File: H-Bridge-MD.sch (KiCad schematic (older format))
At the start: 70 parts, among them IC1 SI8650AB-B-IS1, IC2 AP7381-50SA-7, IC3 A3921KLPTR-T, IC4 SI8650AB-B-IS1, IC5 A3921KLPTR-T, J1 Conn_01x03, J2 Conn_01x05, J3 Bus_mechaken_PCIexpress_x16_1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, J4 Conn_01x02, J5 Conn_01x02, Q1 NVMFD5C446NT1G, Q2 NVMFD5C446NT1G, Q3 NVMFD5C446NT1G, Q4 NVMFD5C446NT1G, U1 LDL1117S33R_SOT223-4, U2 STM32F042K6Tx, U3 MCP2562-E-SN

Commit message: fix
細かな修正
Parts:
- IC2: footprint SamacSys_Parts:SOT96P240X105-3N -> SOT96P240X105-3N; symbol SamacSys_Parts:AP7381-50SA-7 -> H-Bridge-MD-rescue:AP7381-50SA-7-SamacSys_Parts
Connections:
- net MD_3V3 renamed VDD
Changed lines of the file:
@@
 Text GLabel 7600 8550 3    50   Input ~ 0
 MD_FF2_1
-Text GLabel 12750 4150 0    50   Output ~ 0
-MD_3V3
 Text Label 4800 3600 0    50   ~ 0
 CAN_TD
@@
 	0    -1   -1   0
 $EndComp
-Text GLabel 10250 3900 2    50   Input ~ 0
-MD_3V3
-Text GLabel 6050 7450 2    50   Input ~ 0
-MD_3V3
 Connection ~ 9850 10100
 Wire Wire Line
@@
 	1    0    0    -1
 $EndComp
-Text GLabel 11200 4100 3    50   Output ~ 0
-MD_3V3
 Text GLabel 11050 5100 1    50   Input ~ 0
 VREG_0
@@
 Connection ~ 11850 5000
 $Comp
-L SamacSys_Parts:AP7381-50SA-7 IC2
+L H-Bridge-MD-rescue:AP7381-50SA-7-SamacSys_Parts IC2
 U 1 1 5E271866
 P 13300 4050
 F 0 "IC2" H 13850 4315 50  0000 C CNN
 F 1 "AP7381-50SA-7" H 13850 4224 50  0000 C CNN
-F 2 "SamacSys_Parts:SOT96P240X105-3N" H 14250 4150 50  0001 L CNN
+F 2 "SOT96P240X105-3N" H 14250 4150 50  0001 L CNN
 F 3 "https://componentsearchengine.com/Datasheets/1/AP7381-50SA-7.pdf" H 14250 4050 50  0001 L CNN
 F 4 "LDO Voltage Regulators LDO CMOS LowCurr SOT23 T&R 3K" H 14250 3950 50  0001 L CNN "Description"
@@
 Wire Wire Line
 	13100 4450 14400 4450
-Wire Wire Line
-	14400 4450 14400 4050
 Connection ~ 14400 4450
+Wire Wire Line
+	14400 4050 14400 4450
+$Comp
+L power:VDD #PWR0101
+U 1 1 5E33BBA2
+P 11200 4100
+F 0 "#PWR0101" H 11200 3950 50  0001 C CNN
+F 1 "VDD" H 11217 4273 50  0000 C CNN
+F 2 "" H 11200 4100 50  0001 C CNN
+F 3 "" H 11200 4100 50  0001 C CNN
+	1    11200 4100
+	-1   0    0    1
+$EndComp
+$Comp
+L power:VDD #PWR0102
+U 1 1 5E35E290
+P 12750 4150
+F 0 "#PWR0102" H 12750 4000 50  0001 C CNN
+F 1 "VDD" H 12767 4323 50  0000 C CNN
+F 2 "" H 12750 4150 50  0001 C CNN
+F 3 "" H 12750 4150 50  0001 C CNN
+	1    12750 4150
+	0    -1   -1   0
+$EndComp
+$Comp
+L power:VDD #PWR0103
+U 1 1 5E3654B8
+P 10250 3900
+F 0 "#PWR0103" H 10250 3750 50  0001 C CNN
+F 1 "VDD" H 10267 4073 50  0000 C CNN
+F 2 "" H 10250 3900 50  0001 C CNN
+F 3 "" H 10250 3900 50  0001 C CNN
+	1    10250 3900
+	1    0    0    -1
+$EndComp
+$Comp
+L power:VDD #PWR0104
+U 1 1 5E36C54F
+P 6050 7450
+F 0 "#PWR0104" H 6050 7300 50  0001 C CNN
+F 1 "VDD" H 6067 7623 50  0000 C CNN
+F 2 "" H 6050 7450 50  0001 C CNN
+F 3 "" H 6050 7450 50  0001 C CNN
+	1    6050 7450
+	1    0    0    -1
+$EndComp
 $EndSCHEMATC

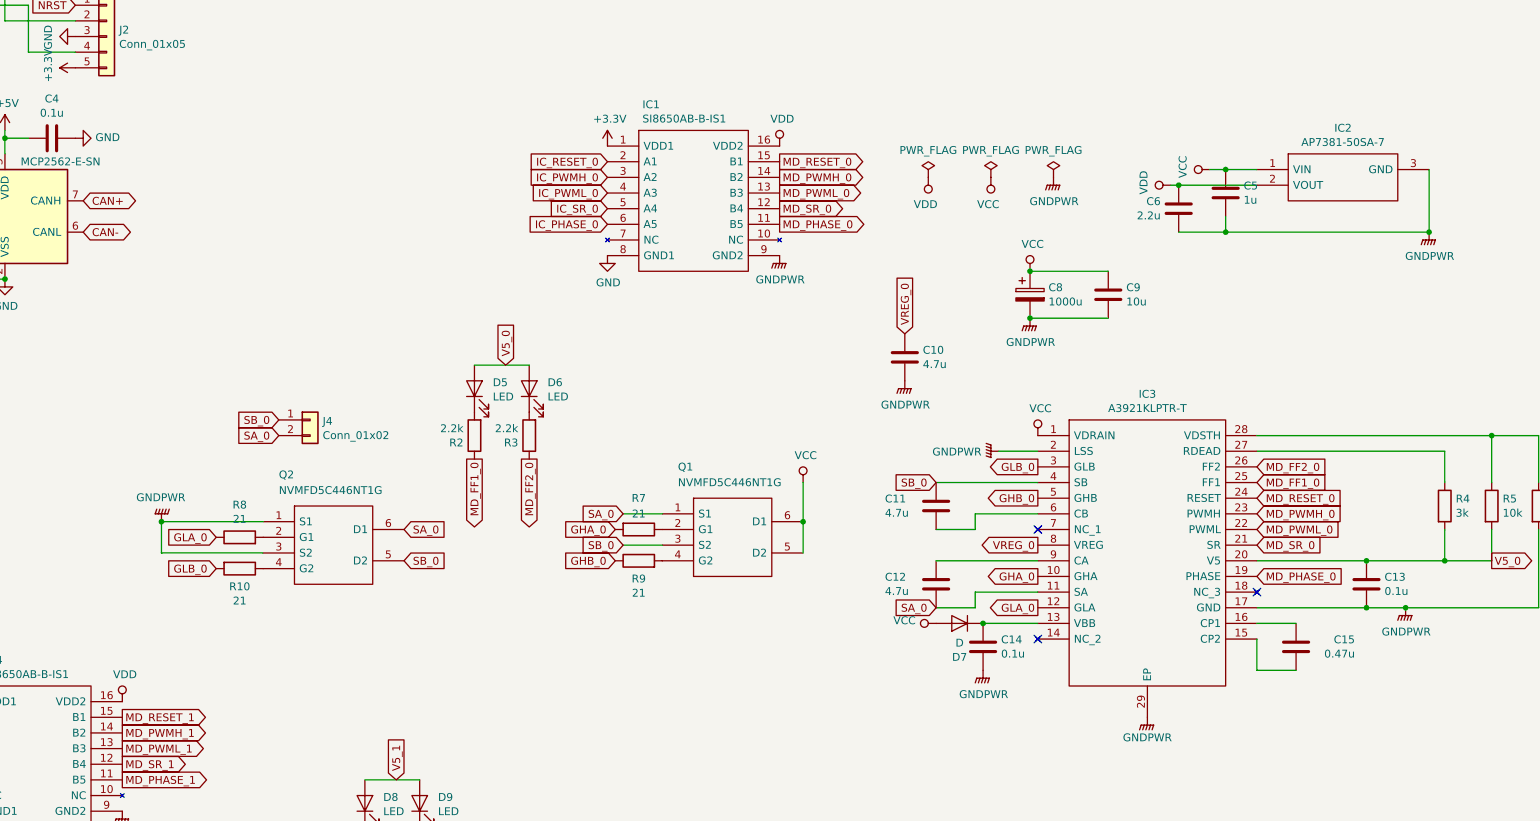
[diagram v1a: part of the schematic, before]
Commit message: clean
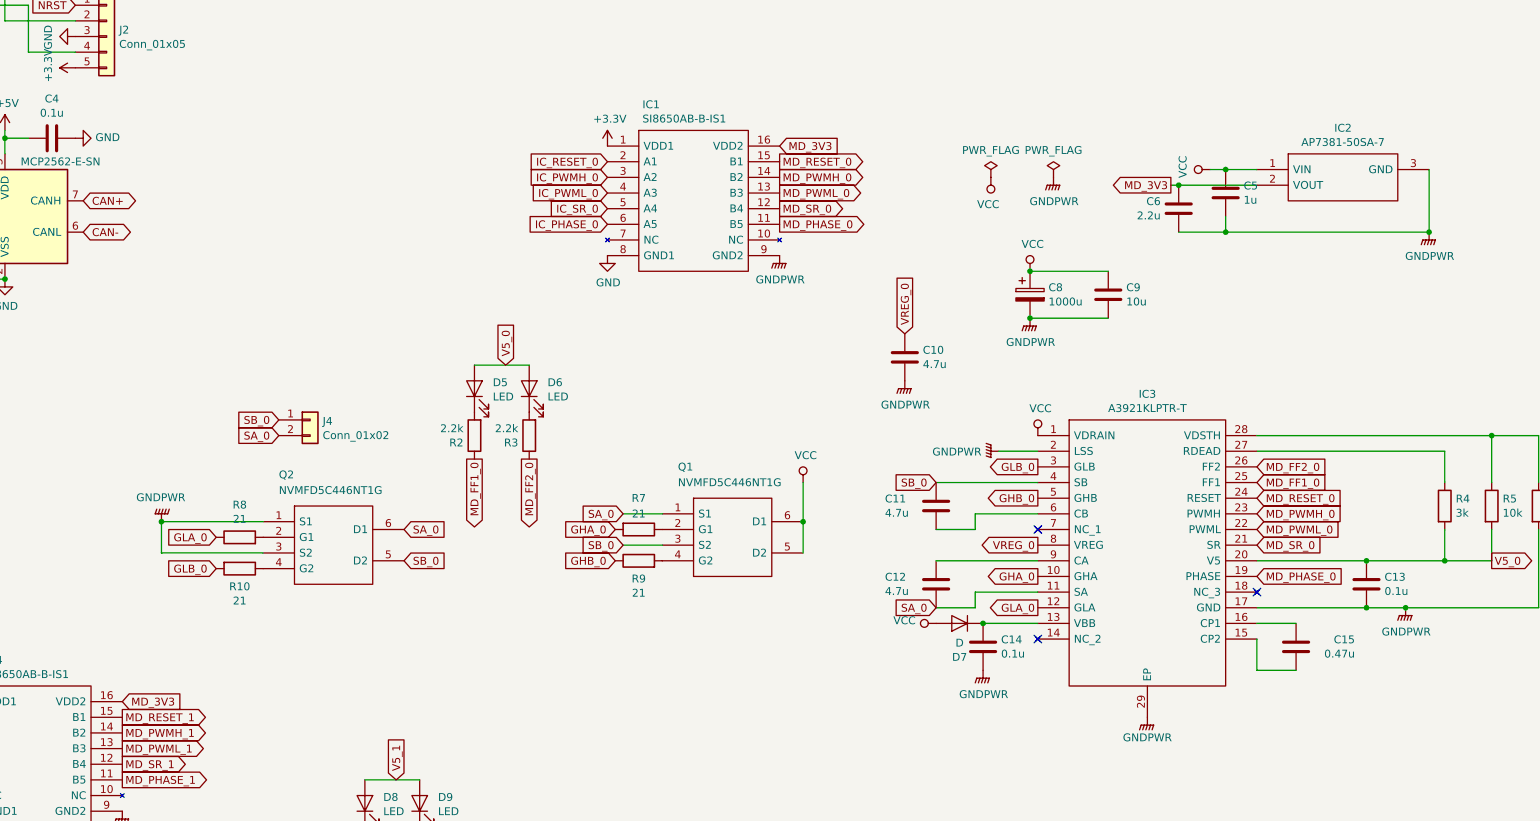
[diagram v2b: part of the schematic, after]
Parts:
- removed IC2: AP7381-50SA-7, SOT96P240X105-3N, symbol H-Bridge-MD-rescue:AP7381-50SA-7-SamacSys_Parts
- added IC2: AP7381-50SA-7, SOT96P240X105-3N, symbol SamacSys_Parts:AP7381-50SA-7
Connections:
- net GNDPWR: now also IC2.3 (GND)
- net VCC: now also IC2.1 (VIN)
- net VDD renamed MD_3V3
- net MD_3V3: now also IC2.2 (VOUT)
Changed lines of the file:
@@
 Text GLabel 7600 8550 3    50   Input ~ 0
 MD_FF2_1
+Text GLabel 12750 4150 0    50   Output ~ 0
+MD_3V3
 Text Label 4800 3600 0    50   ~ 0
 CAN_TD
@@
 	0    -1   -1   0
 $EndComp
+Text GLabel 10250 3900 2    50   Input ~ 0
+MD_3V3
+Text GLabel 6050 7450 2    50   Input ~ 0
+MD_3V3
 Connection ~ 9850 10100
 Wire Wire Line
@@
 F 3 "" H 12000 4050 50  0001 C CNN
 	1    12000 4100
-	1    0    0    -1
-$EndComp
-$Comp
-L power:PWR_FLAG #FLG04
-U 1 1 5E1278AA
-P 11200 4100
-F 0 "#FLG04" H 11200 4175 50  0001 C CNN
-F 1 "PWR_FLAG" H 11200 4273 50  0000 C CNN
-F 2 "" H 11200 4100 50  0001 C CNN
-F 3 "~" H 11200 4100 50  0001 C CNN
-	1    11200 4100
 	1    0    0    -1
 $EndComp
@@
 Connection ~ 11850 5000
 $Comp
-L H-Bridge-MD-rescue:AP7381-50SA-7-SamacSys_Parts IC2
-U 1 1 5E271866
+L Device:C C5
+U 1 1 5DF18189
+P 13100 4200
+F 0 "C5" H 13215 4246 50  0000 L CNN
+F 1 "1u" H 13215 4155 50  0000 L CNN
+F 2 "Capacitor_SMD:C_0805_2012Metric" H 13138 4050 50  0001 C CNN
+F 3 "~" H 13100 4200 50  0001 C CNN
+	1    13100 4200
+	1    0    0    -1
+$EndComp
+Wire Wire Line
+	13300 4050 13100 4050
+Connection ~ 13100 4050
+Wire Wire Line
+	13100 4050 13000 4050
+Wire Wire Line
+	12750 4150 12800 4150
+Connection ~ 12800 4150
+Wire Wire Line
+	12800 4150 13300 4150
+Wire Wire Line
+	12800 4450 13100 4450
+Wire Wire Line
+	13100 4350 13100 4450
+Connection ~ 13100 4450
+Wire Wire Line
+	13100 4450 14400 4450
+Wire Wire Line
+	14400 4450 14400 4050
+Connection ~ 14400 4450
+$Comp
+L SamacSys_Parts:AP7381-50SA-7 IC2
+U 1 1 5E358498
 P 13300 4050
 F 0 "IC2" H 13850 4315 50  0000 C CNN
@@
 	1    0    0    -1
 $EndComp
-$Comp
-L Device:C C5
-U 1 1 5DF18189
-P 13100 4200
-F 0 "C5" H 13215 4246 50  0000 L CNN
-F 1 "1u" H 13215 4155 50  0000 L CNN
-F 2 "Capacitor_SMD:C_0805_2012Metric" H 13138 4050 50  0001 C CNN
-F 3 "~" H 13100 4200 50  0001 C CNN
-	1    13100 4200
-	1    0    0    -1
-$EndComp
-Wire Wire Line
-	13300 4050 13100 4050
-Connection ~ 13100 4050
-Wire Wire Line
-	13100 4050 13000 4050
-Wire Wire Line
-	12750 4150 12800 4150
-Connection ~ 12800 4150
-Wire Wire Line
-	12800 4150 13300 4150
-Wire Wire Line
-	12800 4450 13100 4450
-Wire Wire Line
-	13100 4350 13100 4450
-Connection ~ 13100 4450
-Wire Wire Line
-	13100 4450 14400 4450
-Connection ~ 14400 4450
-Wire Wire Line
-	14400 4050 14400 4450
-$Comp
-L power:VDD #PWR0101
-U 1 1 5E33BBA2
-P 11200 4100
-F 0 "#PWR0101" H 11200 3950 50  0001 C CNN
-F 1 "VDD" H 11217 4273 50  0000 C CNN
-F 2 "" H 11200 4100 50  0001 C CNN
-F 3 "" H 11200 4100 50  0001 C CNN
-	1    11200 4100
-	-1   0    0    1
-$EndComp
-$Comp
-L power:VDD #PWR0102
-U 1 1 5E35E290
-P 12750 4150
-F 0 "#PWR0102" H 12750 4000 50  0001 C CNN
-F 1 "VDD" H 12767 4323 50  0000 C CNN
-F 2 "" H 12750 4150 50  0001 C CNN
-F 3 "" H 12750 4150 50  0001 C CNN
-	1    12750 4150
-	0    -1   -1   0
-$EndComp
-$Comp
-L power:VDD #PWR0103
-U 1 1 5E3654B8
-P 10250 3900
-F 0 "#PWR0103" H 10250 3750 50  0001 C CNN
-F 1 "VDD" H 10267 4073 50  0000 C CNN
-F 2 "" H 10250 3900 50  0001 C CNN
-F 3 "" H 10250 3900 50  0001 C CNN
-	1    10250 3900
-	1    0    0    -1
-$EndComp
-$Comp
-L power:VDD #PWR0104
-U 1 1 5E36C54F
-P 6050 7450
-F 0 "#PWR0104" H 6050 7300 50  0001 C CNN
-F 1 "VDD" H 6067 7623 50  0000 C CNN
-F 2 "" H 6050 7450 50  0001 C CNN
-F 3 "" H 6050 7450 50  0001 C CNN
-	1    6050 7450
-	1    0    0    -1
-$EndComp
